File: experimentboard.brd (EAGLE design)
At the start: 152.4 x 100 mm, 160 parts, among them IC1 TL072P, IC2 LM317, IC3 LM337, IC4 TL072P, IC5 TL072P, IC6 TL072P, U1 PCM1690, U2 DIR9001

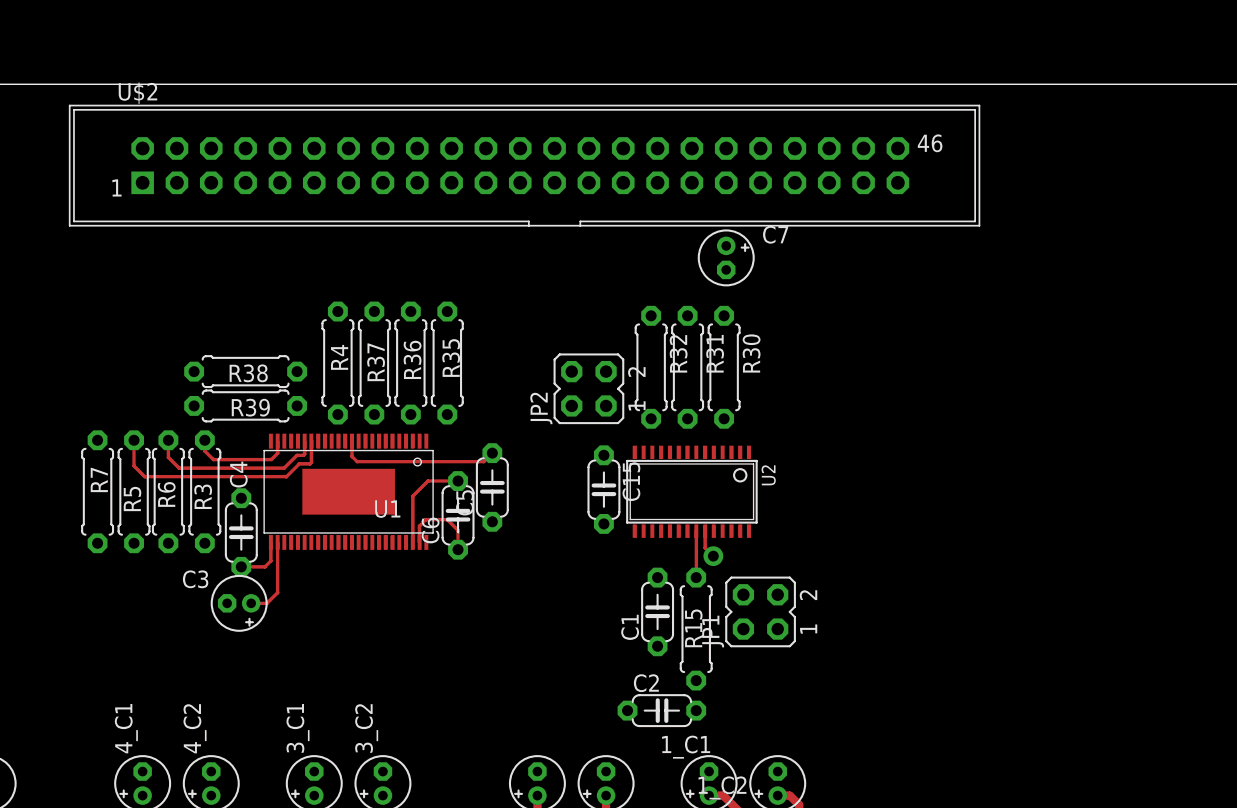
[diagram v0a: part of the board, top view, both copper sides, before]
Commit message: Working on EEPROM and TOSLINK
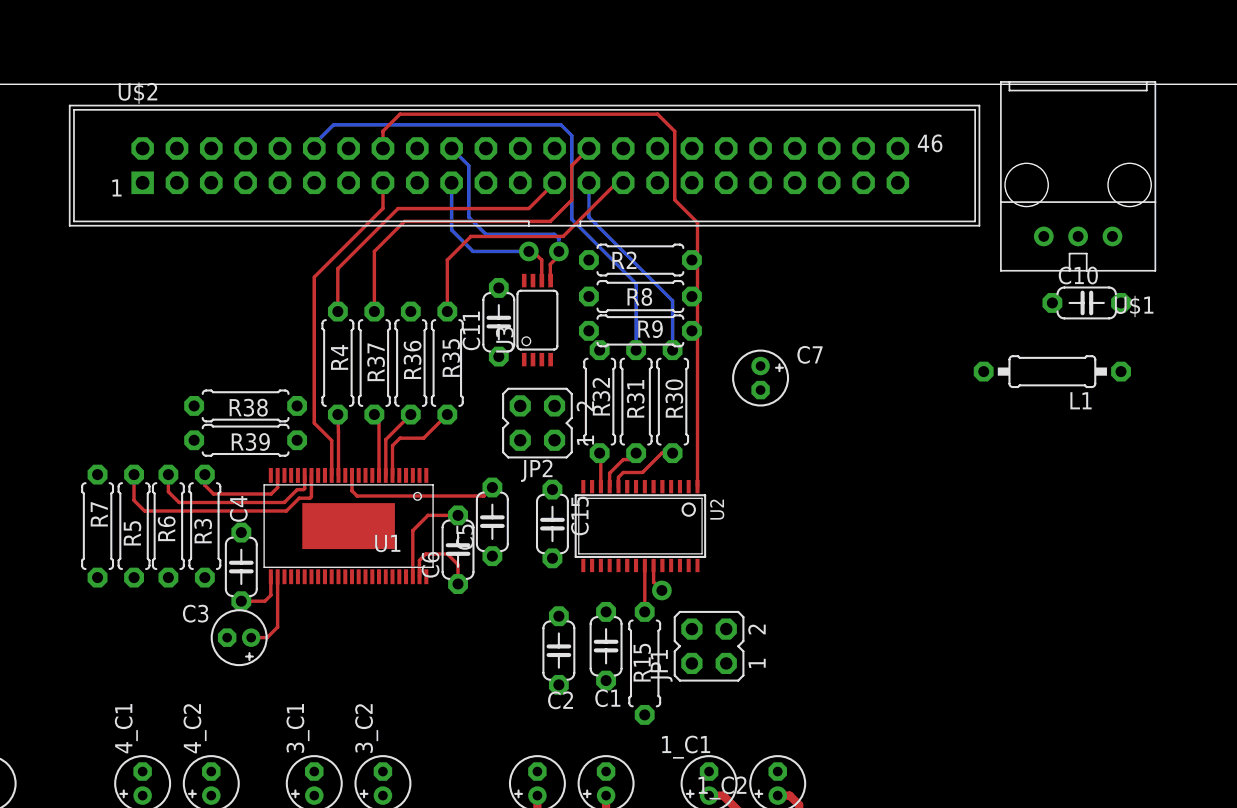
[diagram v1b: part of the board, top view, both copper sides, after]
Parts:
- added C10, C11: 100nf, rcl:C050-024X044
- added L1: 47uH, rcl:0207/10
- added R2, R8, R9: 5.6k, rcl:0207/7
- added U$1: PLR135/T9, 0000halfgaar:PLR135/T9
- added U3: CAT24C256, 0000halfgaar:TSSOP8
- moved C7 9.25 mm to (113.0, 78.3)
- moved C2 8.82 mm to (98.1, 58.1), turned to 270 degrees
- moved C15 4.58 mm to (97.6, 67.5)
- moved R30 4.58 mm to (106.5, 76.5)
- moved R32 4.58 mm to (101.1, 76.5)
- moved C1 4.58 mm to (101.6, 58.4)
- moved JP1 4.58 mm to (109.2, 58.4)
- moved R15 4.58 mm to (104.5, 57.1)
- moved JP2 4.58 mm to (96.5, 74.9)
- moved U2 4.58 mm to (104.1, 67.3)
- moved R31 4.58 mm to (103.8, 76.5)
- moved C5 2.54 mm to (93.2, 67.6)
- moved C6 2.54 mm to (90.6, 65.6)
- moved R39 2.54 mm to (74.9, 73.7)
- moved C3 2.54 mm to (74.5, 59.1)
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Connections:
- new net CAPE_I2C_SCL: R8.1, U$2.19, U3.6
- new net CAPE_I2C_SDA: R2.1, U$2.20, U3.5
- net DGND: now also C10.1, C11.1, U$1.2, U3.4
- net N$20: now also U$1.1
- net N$54: now also R9.1, U3.3; no longer U2.4
- net VDD: now also C10.2, C11.2, L1.1, L1.2, R2.2, R8.2, R9.2, U$1.3, U3.8
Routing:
- net DIR_AUDIO: track 0.00 -> 50.9 mm
- net ACLKR: track 0.00 -> 38.1 mm
- net DOUT: track 0.00 -> 25.0 mm
- net RST: track 0.00 -> 24.3 mm
- net MCLK: track 0.00 -> 21.8 mm
- net AHCLKX: track 0.00 -> 19.2 mm
- net CAPE_I2C_SDA: track 0.00 -> 16.3 mm, vias 0 -> 1
- net FSR: track 0.00 -> 14.9 mm
- net CAPE_I2C_SCL: track 0.00 -> 12.6 mm, vias 0 -> 1
- net N$63: track 0.00 -> 7.21 mm
- net N$53: track 0.00 -> 5.44 mm
- net N$62: track 0.00 -> 5.27 mm
- net N$61: track 0.00 -> 4.65 mm
- net N$5: track 0.00 -> 4.51 mm
- net N$52: track 0.00 -> 3.57 mm
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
